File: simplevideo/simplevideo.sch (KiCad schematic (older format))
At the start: 9 parts, among them J1 Conn_01x02, Q2 2N3904, U2 74LS08

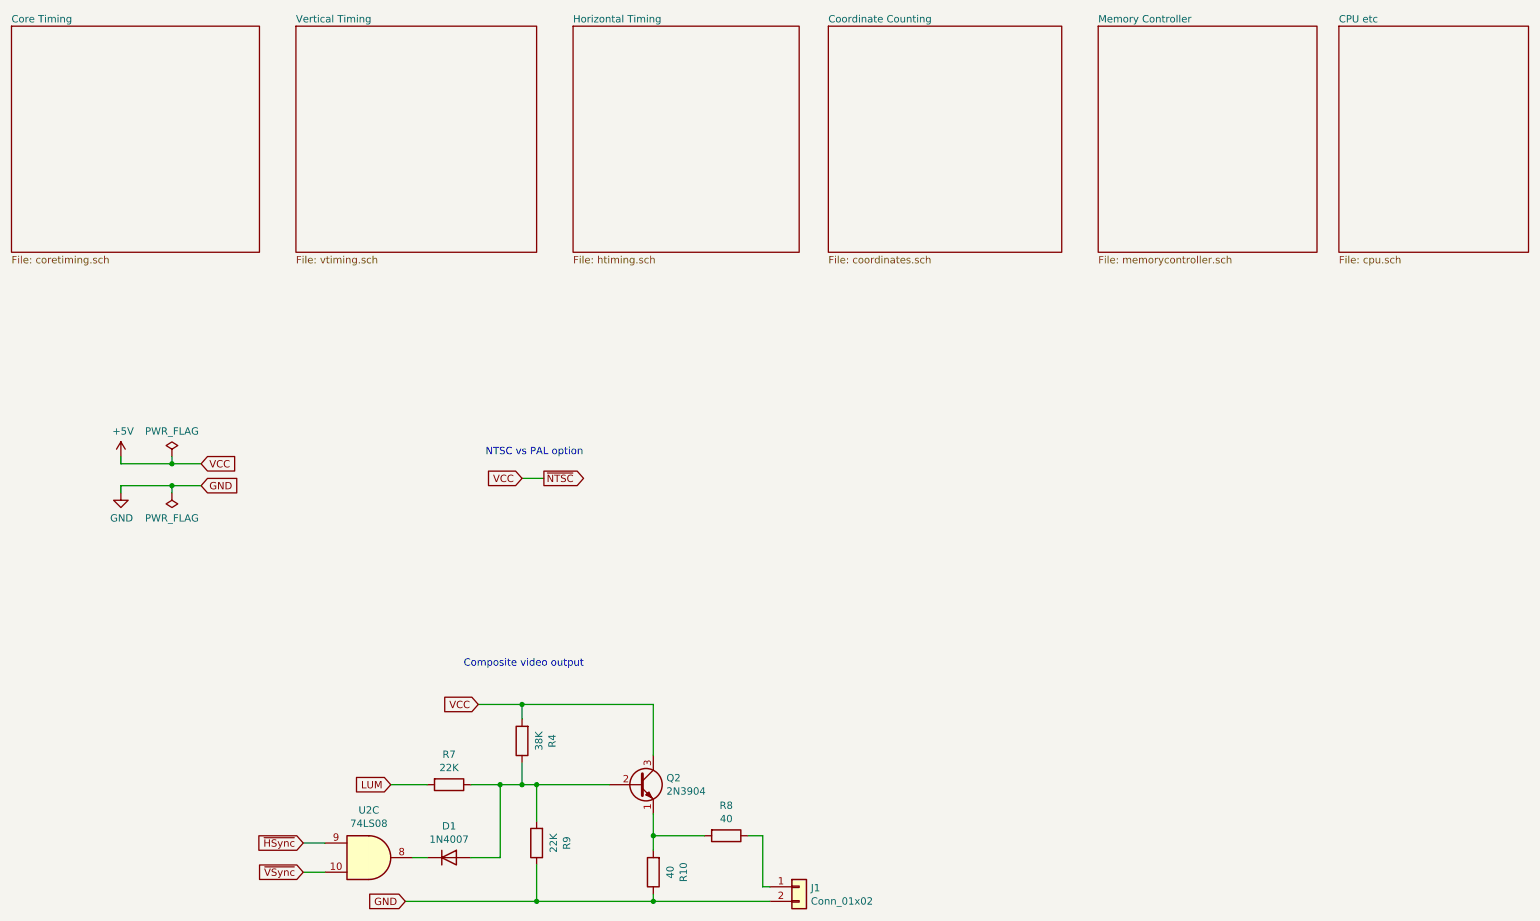
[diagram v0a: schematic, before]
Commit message: Fixed various issues discovered during building and testing
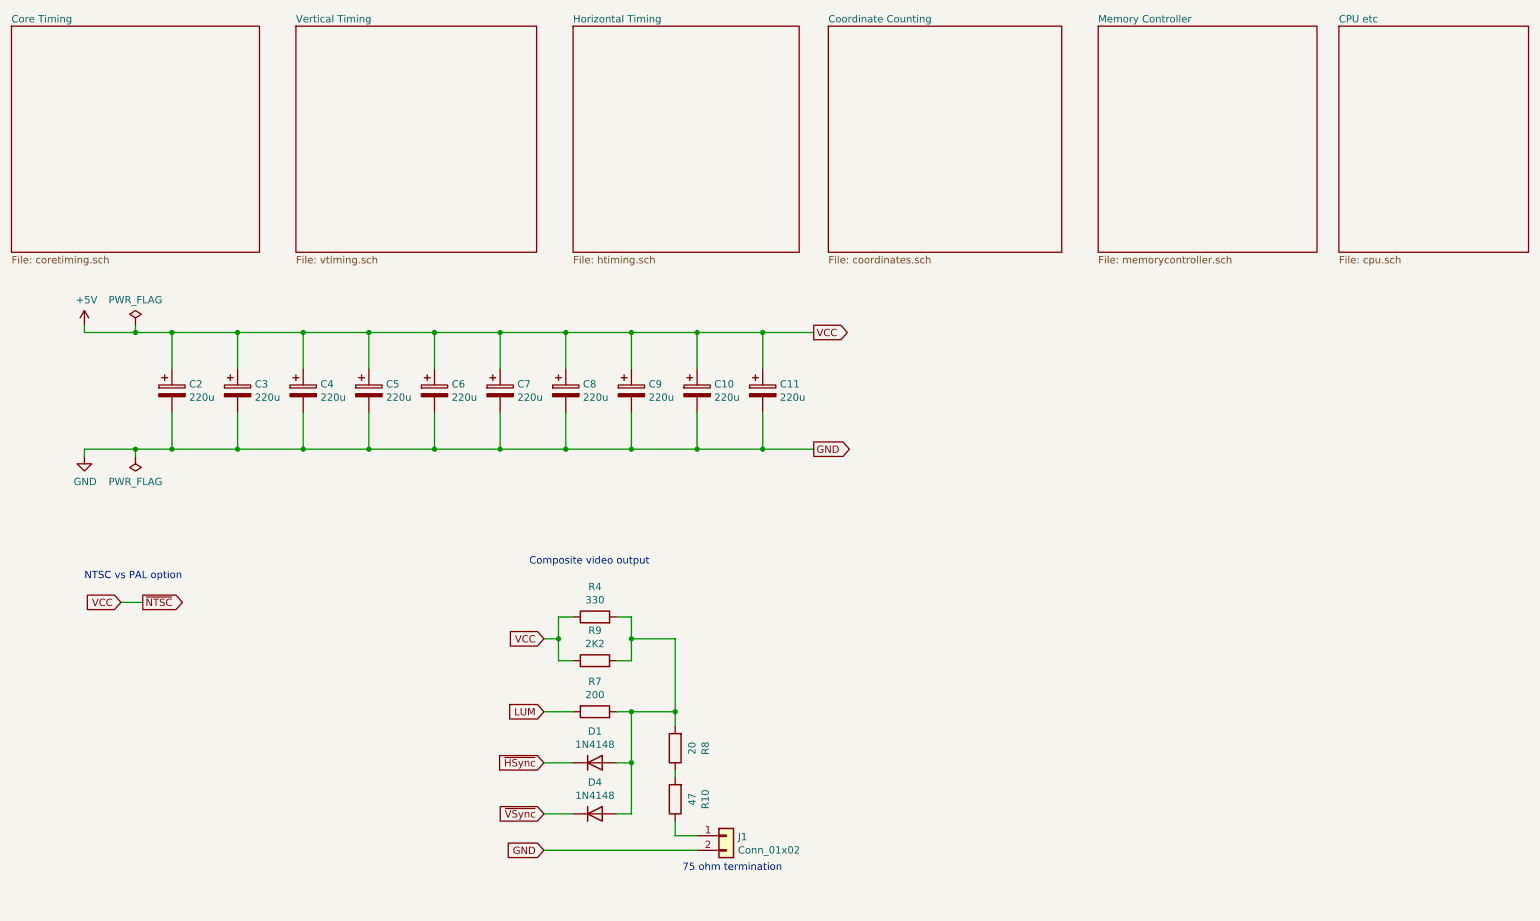
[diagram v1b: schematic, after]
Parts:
- removed Q2: 2N3904, Package_TO_SOT_THT:TO-92_Inline, symbol Transistor_BJT:2N3904
- removed U2: 74LS08, Package_DIP:DIP-14_W7.62mm, symbol 74xx:74LS08
- added C10, C11, C2, C3, C4, C5, C6, C7, C8, C9: 220u, Capacitor_THT:CP_Radial_D5.0mm_P2.50mm, symbol Device:CP
- added D4: 1N4148, Diode_THT:D_DO-34_SOD68_P7.62mm_Horizontal, symbol Diode:1N4007
- D1: value 1N4007 -> 1N4148
- R10: value 40 -> 47
- R4: value 38K -> 330
- R7: value 22K -> 200
- R8: value 40 -> 20
- R9: value 22K -> 2K2
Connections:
- net +5V: now also R4.1, R9.1, C10.1, C11.1, C2.1, C3.1, C4.1, C5.1, C6.1, C7.1, C8.1, C9.1; no longer R4.2
- net GND: now also C10.2, C11.2, C2.2, C3.2, C4.2, C5.2, C6.2, C7.2, C8.2, C9.2; no longer R10.1, R9.1
- net ~HSync: now also D1.1 (K)
- net ~VSync: now also D4.1 (K)
- net at R10.2: now also R8.1; no longer R8.2
- net at J1.1 (Pin_1): now also R10.1; no longer R8.1
- net at D1.2 (A), R7.1, R9.2: now also R4.2, R8.2, D4.2 (A); no longer R4.1
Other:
- note added: "75 ohm termination"
- moved on the sheet: D1, J1, R4, R7, R8
